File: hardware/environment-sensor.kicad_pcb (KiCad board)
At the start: 2 copper layers, 100 x 84 mm, 112 parts, among them J1 J1B1211CCD, P1 USB_OTG, P2 ICSP, P3 JTAG, P4 NSL-19M51, P5 PPD42, P6 POWER, SW1 Reset, U1 ATMEGA32U4-AU, U2 W5500, U3 Bosch_BME280, U4 LT1761-5, U5 LT1761-3.3, X1 16MHz, X2 25MHz

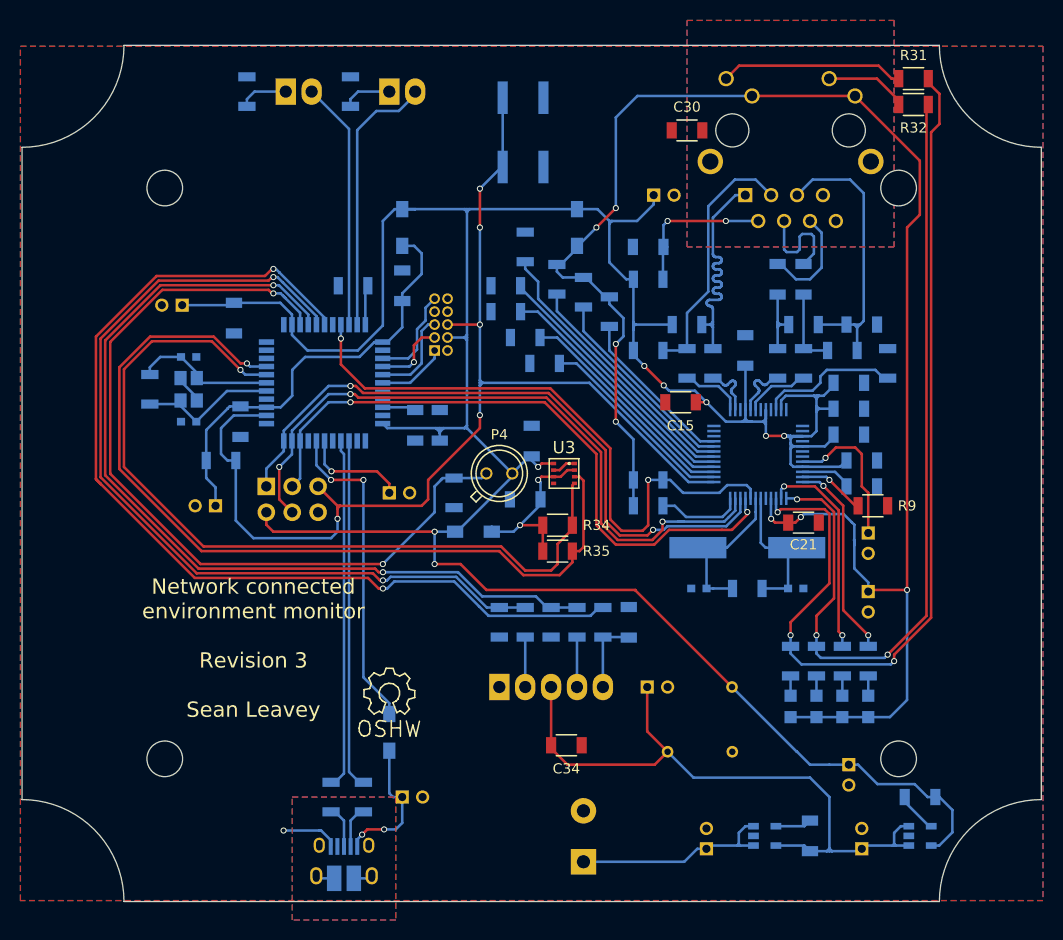
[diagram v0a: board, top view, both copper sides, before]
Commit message: New revision to board
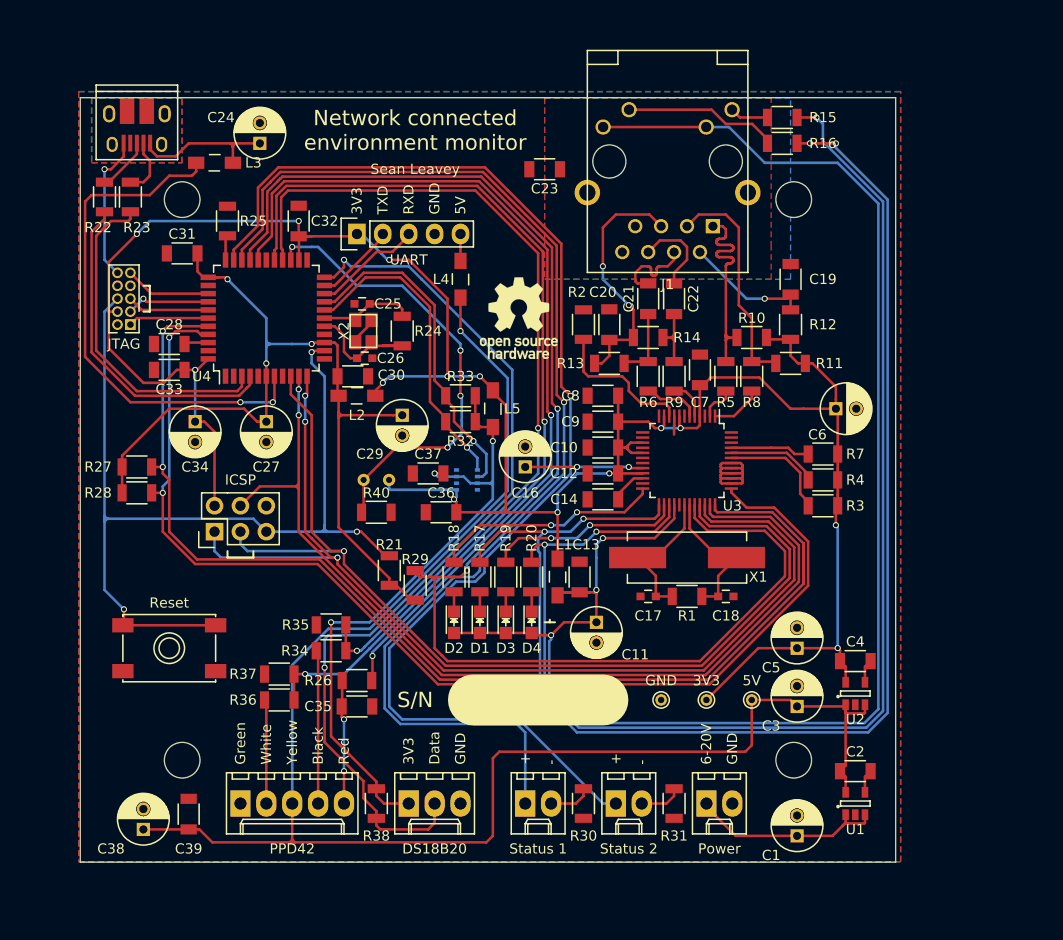
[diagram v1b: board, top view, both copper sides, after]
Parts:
- removed C15: 100n, Capacitors_SMD:C_1206
- removed D5: DUPLED, LEDs:LED_0805
- removed D6: ACTLED, LEDs:LED_0805
- removed R41, R42, R43: 330R, Resistors_SMD:R_1206
- removed REF**: Symbol_OSHW-Logo_SilkScreen, Symbols:Symbol_OSHW-Logo_SilkScreen
- removed the Ref** at (156.8, 101.0)
- added L5: Wurth WE-CBF, Choke_SMD:Choke_SMD_1206_Standard, F.Cu at (153.0, 94.6)
- added P7: JTAG, Pin_Headers:Pin_Header_Straight_2x05_Pitch1.27mm, F.Cu at (117.5, 86.4)
- added P8: DS18B20, Connectors_Molex:Molex_KK-6410-03_03x2.54mm_Straight, F.Cu at (144.8, 133.3)
- added P9: PPD42, Connectors_Molex:Molex_KK-6410-05_05x2.54mm_Straight, F.Cu at (128.3, 133.3)
- added REF***: OSHW-Logo_7.5x8mm_SilkScreen, Symbols:OSHW-Logo_7.5x8mm_SilkScreen, F.Cu at (155.6, 85.7)
- added Ref**: Val**, Board_Outlines:80mmx75mm_holes, F.Cu at (152.6, 101.6)
- C1, C10, C11, C12, C31, C32, C6, C7, C8, C9, L1, L2, L3, L4, R21, R36, R37, W1, W2, W3: moved to F.Cu
- C13, C33, C35, C37, C39: value 10u -> 100n; footprint Capacitors_ThroughHole:C_Radial_D5_L11_P2 -> Capacitors_SMD:C_1206; moved to F.Cu
- C14, C20: value 100n -> 10n; moved to F.Cu
- C16: value 100n -> 4u7; footprint Capacitors_SMD:C_1206 -> Capacitors_ThroughHole:C_Radial_D5_L11_P2; moved to F.Cu
- C17: value 100n -> 32p; footprint Capacitors_SMD:C_1206 -> Capacitors_SMD:C_0603; moved to F.Cu
- C18: value 10u -> 32p; footprint Capacitors_ThroughHole:C_Radial_D5_L11_P2 -> Capacitors_SMD:C_0603; moved to F.Cu
- C19: value 100n -> 22n; moved to F.Cu
- C2: value 12p -> 10n; footprint Capacitors_SMD:C_0603 -> Capacitors_SMD:C_1206; moved to F.Cu
- C21: value 100n -> 6.8n
- C22: value 10n -> 6.8n; moved to F.Cu
- C23: value 4u7 -> 1n/2kV; footprint Capacitors_ThroughHole:C_Radial_D5_L11_P2 -> Capacitors_SMD:C_1206; moved to F.Cu
- C24: value 32p -> 10u; footprint Capacitors_SMD:C_0603 -> Capacitors_ThroughHole:C_Radial_D5_L11_P2; moved to F.Cu
- C25: value 32p -> 12p; moved to F.Cu
- C26: value 22n -> 12p; footprint Capacitors_SMD:C_1206 -> Capacitors_SMD:C_0603; moved to F.Cu
- C27: value 10n -> 1u; footprint Capacitors_SMD:C_1206 -> Capacitors_ThroughHole:C_Radial_D5_L11_P2; moved to F.Cu
- C28: value 6.8n -> 100n; moved to F.Cu
- C29: value 6.8n -> 10u; footprint Capacitors_SMD:C_1206 -> Capacitors_ThroughHole:C_Radial_D5_L11_P2; moved to F.Cu
- C3: value 12p -> 10u; footprint Capacitors_SMD:C_0603 -> Capacitors_ThroughHole:C_Radial_D5_L11_P2; moved to F.Cu
- C30: value 1n/2kV -> 100n
- C34: value 100n -> 10u; footprint Capacitors_SMD:C_1206 -> Capacitors_ThroughHole:C_Radial_D5_L11_P2
- C36: value 10n -> 100n; moved to F.Cu
- C38: value 10n -> 10u; footprint Capacitors_SMD:C_1206 -> Capacitors_ThroughHole:C_Radial_D5_L11_P2; moved to F.Cu
- C4: value 1u -> 10n; footprint Capacitors_ThroughHole:C_Radial_D5_L11_P2 -> Capacitors_SMD:C_1206; moved to F.Cu
- C5: value 100n -> 10u; footprint Capacitors_SMD:C_1206 -> Capacitors_ThroughHole:C_Radial_D5_L11_P2; moved to F.Cu
- D1: value Status 1 -> LINKLED; footprint Connectors_Molex:Molex_KK-6410-02_02x2.54mm_Straight -> LEDs:LED_0805; moved to F.Cu
- D2: value Status 2 -> SPDLED; footprint Connectors_Molex:Molex_KK-6410-02_02x2.54mm_Straight -> LEDs:LED_0805; moved to F.Cu
- D3: value LINKLED -> DUPLED; moved to F.Cu
- D4: value SPDLED -> ACTLED; moved to F.Cu
- J1: footprint Cetus_RJ45:Cetus_J1B1211CCD -> Sockets_RJ45:Cetus_J1B1211CCD; moved to F.Cu
- P1: value USB_OTG -> POWER; footprint Connect:USB_Micro-B_10103594-0001LF -> Connectors_Molex:Molex_KK-6410-02_02x2.54mm_Straight; moved to F.Cu
- P2: value ICSP -> USB_OTG; footprint Pin_Headers:Pin_Header_Straight_2x03 -> Connect:USB_Micro-B_10103594-0001LF; moved to F.Cu
- P3: value JTAG -> ICSP; footprint Pin_Headers:Pin_Header_Straight_2x05_Pitch1.27mm -> Pin_Headers:Pin_Header_Straight_2x03; moved to F.Cu
- P4: value NSL-19M51 -> STATUS 1; footprint TO_SOT_Packages_THT:TO-18_2Pin -> Connectors_Molex:Molex_KK-6410-02_02x2.54mm_Straight
- P5: value PPD42 -> STATUS 2; footprint Connectors_Molex:Molex_KK-6410-05_05x2.54mm_Straight -> Connectors_Molex:Molex_KK-6410-02_02x2.54mm_Straight; moved to F.Cu
- P6: value POWER -> UART; footprint Terminal_Blocks:TerminalBlock_Pheonix_MKDS1.5-2pol -> Pin_Headers:Pin_Header_Straight_1x05; moved to F.Cu
- R1: value 10k -> 1M; moved to F.Cu
- R10, R11, R14: value 10k -> 49R9; moved to F.Cu
- R12: value 1M -> 10R; moved to F.Cu
- R13: value 12k4/1% -> 49R9; moved to F.Cu
- R15, R18, R19, R20: value 10k -> 330R; moved to F.Cu
- R16, R17: value 0R -> 330R; moved to F.Cu
- R2: value 22R -> 12k4/1%; moved to F.Cu
- R22, R23: value 10k -> 22R; moved to F.Cu
- R24: value 0R -> 1M; moved to F.Cu
- R25: value 0R -> 10k; moved to F.Cu
- R26, R27, R29: value 49R9/1% -> 10k; moved to F.Cu
- R28: value 10R/1% -> 10k; moved to F.Cu
- R3: value 22R -> 10k; moved to F.Cu
- R30: value 49R9/1% -> 180R; moved to F.Cu
- R31: value 330R -> 180R
- R32: value 330R -> 4k7
- R33, R38: value 10k -> 4k7; moved to F.Cu
- R34, R35: value 4k7 -> 10k
- R39: value 10k -> NSL-19M51; footprint Resistors_SMD:R_1206 -> LDRs_NSL:NSL_19M51
- R4: value 1M -> 10k; moved to F.Cu
- R40: value 330R -> 10k; moved to F.Cu
- R5, R8: value 10k -> 0R; moved to F.Cu
- R6: value 180R -> 0R; moved to F.Cu
- R7: value 180R -> 10k; moved to F.Cu
- R9: value 10k -> 0R
- SW1: value Reset -> RESET; footprint Buttons_Switches_SMD:SW_SPST_EVQP0 -> Buttons_Switches_SMD_FSM_JSM:SW_SPST_FSM_JSM; moved to F.Cu
- U1: value ATMEGA32U4-AU -> LT1761-5; footprint Housings_QFP:TQFP-44_10x10mm_Pitch0.8mm -> TO_SOT_Packages_SMD:SOT-23-5; moved to F.Cu
- U2: value W5500 -> LT1761-3.3; footprint Housings_QFP:LQFP-48_7x7mm_Pitch0.5mm -> TO_SOT_Packages_SMD:SOT-23-5; moved to F.Cu
- U3: value Bosch_BME280 -> W5500; footprint Bosch_Environment_Sensor:Bosch_BME280_LGA-8 -> Housings_QFP:LQFP-48_7x7mm_Pitch0.5mm
- U4: value LT1761-5 -> ATMEGA32U4-AU; footprint TO_SOT_Packages_SMD:SOT-23-5 -> Housings_QFP:TQFP-44_10x10mm_Pitch0.8mm; moved to F.Cu
- U5: value LT1761-3.3 -> Bosch_BME280; footprint TO_SOT_Packages_SMD:SOT-23-5 -> Sensors_LGA:Bosch_BME280_LGA-8
- X1: value 16MHz -> 25MHz; footprint Crystals:crystal_FA238-TSX3225 -> Crystals:Crystal_HC49-SD_SMD; moved to F.Cu
- X2: value 25MHz -> 16MHz; footprint Crystals:Crystal_HC49-SD_SMD -> Crystals:crystal_FA238-TSX3225; moved to F.Cu
- moved C2 77.0 mm to (188.6, 130.2), turned to 180 degrees
- moved C38 76.3 mm to (118.7, 135.9), turned to 90 degrees
- moved R31 74.9 mm to (170.8, 133.3), turned to 90 degrees
- moved U4 70.5 mm to (130.8, 85.7), turned to 90 degrees
- moved C24 68.3 mm to (130.2, 68.6), turned to 90 degrees
- moved R4 66.6 mm to (185.4, 101.6), turned to 180 degrees
- moved U1 66.4 mm to (188.6, 133.3)
- moved C3 65.9 mm to (182.9, 123.8), turned to 90 degrees
- moved P6 65.5 mm to (139.7, 77.5)
- moved C39 65.0 mm to (123.2, 134.4)
- moved C28 62.6 mm to (121.3, 88.3), turned to 180 degrees
- moved C6 61.6 mm to (186.7, 94.6), turned to 0 degrees
- moved SW1 61.4 mm to (121.3, 118.1), turned to 0 degrees
- moved C27 59.2 mm to (130.8, 95.9), turned to 270 degrees
- moved R7 58.4 mm to (185.4, 99.1), turned to 180 degrees
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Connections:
- C1 pad 1: Net-(C1-Pad1) -> /Power Supply/+6V
- C10 pad 1: GND -> /Microcontroller/3V3A
- C10 pad 2: /Microcontroller/3V3A -> GND
- C11 pad 1: /Microcontroller/3V3A -> /Network I/O/3V3D
- C12 pad 1: /Microcontroller/P_THRESH -> /Microcontroller/3V3A
- C13 pad 1: /Microcontroller/3V3A -> /Network I/O/3V3D
- C14 pad 1: /Microcontroller/3V3A -> GND
- C14 pad 2: GND -> Net-(C14-Pad2)
- C16 pad 1: /Microcontroller/3V3A -> Net-(C16-Pad1)
- C17 pad 1: /Microcontroller/3V3A -> GND
- C17 pad 2: GND -> Net-(C17-Pad2)
- C18 pad 1: /Network I/O/3V3D -> GND
- C18 pad 2: GND -> Net-(C18-Pad2)
- C19 pad 1: /Microcontroller/3V3A -> Net-(C19-Pad1)
- C2 pad 2: GND -> /Microcontroller/5VA
- C20 pad 1: /Microcontroller/3V3A -> Net-(C20-Pad1)
- C21 pad 1: /Network I/O/3V3D -> /Network I/O/RX2+
- C21 pad 2: GND -> /Network I/O/RX1+
- C22 pad 1: GND -> /Network I/O/RX2-
- C22 pad 2: Net-(C22-Pad2) -> /Network I/O/RX1-
- C23 pad 1: Net-(C23-Pad1) -> GND
- C23 pad 2: GND -> /Network I/O/CHGND
- C24 pad 1: GND -> Net-(C24-Pad1)
- C24 pad 2: Net-(C24-Pad2) -> GND
- C25 pad 1: GND -> Net-(C25-Pad1)
- C25 pad 2: Net-(C25-Pad2) -> GND
- C27 pad 1: Net-(C27-Pad1) -> /Microcontroller/3V3D
- C28 pad 1: /Network I/O/RX2+ -> Net-(C28-Pad1)
- C28 pad 2: /Network I/O/RX1+ -> GND
- C29 pad 1: /Network I/O/RX2- -> /Microcontroller/3V3D
- C29 pad 2: /Network I/O/RX1- -> GND
- C3 pad 1: Net-(C3-Pad1) -> /Microcontroller/5VA
- C30 pad 2: /Network I/O/CHGND -> /Microcontroller/3V3D
- C31 pad 1: /Microcontroller/3V3A -> GND
- C31 pad 2: GND -> /Microcontroller/3V3D
- C32 pad 1: /Sensors/3V3D -> GND
- C32 pad 2: GND -> /Microcontroller/3V3A
- C33 pad 1: /Power Supply/5VA -> GND
- C33 pad 2: GND -> /Microcontroller/3V3A
- C34 pad 1: GND -> /Microcontroller/3V3A
- C34 pad 2: /Power Supply/5VA -> GND
- C35 pad 1: /Power Supply/+6V -> /Microcontroller/DUST_2_THRESH
- C36 pad 1: Net-(C36-Pad1) -> /Microcontroller/3V3A
- C36 pad 2: /Power Supply/5VA -> GND
- C37 pad 1: /Power Supply/5VA -> /Sensors/3V3D
- C38 pad 1: Net-(C38-Pad1) -> /Microcontroller/5VA
- C38 pad 2: /Microcontroller/3V3A -> GND
- C39 pad 1: /Microcontroller/3V3A -> GND
- C39 pad 2: GND -> /Microcontroller/5VA
- C4 pad 2: GND -> /Microcontroller/3V3A
- C5 pad 1: Net-(C5-Pad1) -> /Microcontroller/3V3A
- C6 pad 1: /Microcontroller/3V3D -> /Microcontroller/3V3A
- C7 pad 1: GND -> /Microcontroller/3V3A
- C7 pad 2: /Microcontroller/3V3D -> GND
- C8 pad 1: GND -> /Microcontroller/3V3A
- C8 pad 2: /Microcontroller/3V3D -> GND
- C9 pad 1: GND -> /Microcontroller/3V3A
- C9 pad 2: /Microcontroller/3V3A -> GND
- D1 pad 2: Net-(D1-Pad2) -> /Network I/O/3V3D
- D2 pad 2: Net-(D2-Pad2) -> /Network I/O/3V3D
- J1 pad 2: Net-(C26-Pad1) -> Net-(C19-Pad1)
- J1 pad 5: Net-(C27-Pad1) -> Net-(C20-Pad1)
- L1 pad 1: /Microcontroller/3V3A -> /Network I/O/3V3D
- L1 pad 2: /Microcontroller/3V3D -> /Microcontroller/3V3A
- L2 pad 1: Net-(C1-Pad1) -> /Microcontroller/3V3A
- L2 pad 2: Net-(L2-Pad2) -> /Microcontroller/3V3D
- L3 pad 1: /Microcontroller/3V3A -> Net-(C24-Pad1)
- L3 pad 2: /Network I/O/3V3D -> Net-(L3-Pad2)
- L4 pad 1: /Microcontroller/3V3A -> Net-(L4-Pad1)
- L4 pad 2: /Sensors/3V3D -> /Microcontroller/5VA
- P1 pad 1: Net-(C1-Pad1) -> /Power Supply/+6V
- P1 pad 2: /Microcontroller/USBD- -> GND
- P2 pad 1: /Microcontroller/SPI_MISO -> Net-(C24-Pad1)
- P2 pad 2: /Microcontroller/3V3A -> /Microcontroller/USBD-
- P2 pad 3: /Microcontroller/SPI_SCLK -> /Microcontroller/USBD+
- P2 pad 4: /Microcontroller/SPI_MOSI -> (no net)
- P2 pad 5: /Microcontroller/~RESET -> GND
- P2 pad 6: GND -> Net-(P2-Pad6)
- P3 pad 1: Net-(P3-Pad1) -> /Microcontroller/SPI_MISO
- P3 pad 2: GND -> /Microcontroller/3V3A
- P3 pad 3: Net-(P3-Pad3) -> /Microcontroller/SPI_SCLK
- P3 pad 4: /Microcontroller/3V3A -> /Microcontroller/SPI_MOSI
- P3 pad 5: Net-(P3-Pad5) -> /Microcontroller/~RESET
- P3 pad 6: /Microcontroller/~RESET -> GND
- P4 pad 1: /Microcontroller/3V3A -> /Microcontroller/STATUS_1
- P4 pad 2: /Microcontroller/LDR_OUT -> Net-(P4-Pad2)
- P5 pad 1: GND -> /Microcontroller/STATUS_2
- P6 pad 1: /Power Supply/+6V -> /Microcontroller/3V3A
- P6 pad 2: GND -> Net-(P6-Pad2)
- R1 pad 1: /Microcontroller/3V3D -> Net-(C17-Pad2)
- R1 pad 2: /Microcontroller/~RESET -> Net-(C18-Pad2)
- R10 pad 1: /Network I/O/3V3D -> /Network I/O/TX1+
- R10 pad 2: /Microcontroller/SS_PHY -> /Microcontroller/3V3A
- R11 pad 1: /Network I/O/3V3D -> /Network I/O/TX1-
- R11 pad 2: Net-(R11-Pad2) -> /Microcontroller/3V3A
- R12 pad 1: Net-(C24-Pad2) -> Net-(C19-Pad1)
- R12 pad 2: Net-(C25-Pad2) -> /Microcontroller/3V3A
- R13 pad 1: GND -> Net-(C20-Pad1)
- R13 pad 2: Net-(R13-Pad2) -> /Network I/O/RX1+
- R14 pad 1: /Network I/O/3V3D -> Net-(C20-Pad1)
- R14 pad 2: Net-(R14-Pad2) -> /Network I/O/RX1-
- R15 pad 1: /Network I/O/3V3D -> Net-(J1-Pad9)
- R15 pad 2: Net-(R15-Pad2) -> /Network I/O/ACTLED
- R16 pad 1: /Network I/O/TX1+ -> Net-(J1-Pad11)
- R16 pad 2: /Network I/O/TX+ -> /Network I/O/LINKLED
- R17 pad 1: /Network I/O/RX1+ -> Net-(D1-Pad1)
- R17 pad 2: /Network I/O/RX+ -> /Network I/O/LINKLED
- R18 pad 1: GND -> Net-(D2-Pad1)
- R18 pad 2: Net-(R18-Pad2) -> /Network I/O/SPDLED
- R19 pad 1: GND -> Net-(D3-Pad1)
- R19 pad 2: Net-(R19-Pad2) -> /Network I/O/DUPLED
- R2 pad 1: /Microcontroller/USBD1+ -> GND
- R2 pad 2: /Microcontroller/USBD+ -> Net-(R2-Pad2)
- R20 pad 1: GND -> Net-(D4-Pad1)
- R20 pad 2: Net-(R20-Pad2) -> /Network I/O/ACTLED
- R21 pad 1: GND -> /Microcontroller/~RESET
- R21 pad 2: Net-(R21-Pad2) -> /Microcontroller/3V3D
- R22 pad 1: GND -> /Microcontroller/USBD+
- R22 pad 2: Net-(R22-Pad2) -> /Microcontroller/USBD1+
- R23 pad 1: /Network I/O/3V3D -> /Microcontroller/USBD-
- R23 pad 2: Net-(R23-Pad2) -> /Microcontroller/USBD1-
- R24 pad 1: /Network I/O/TX1- -> Net-(C26-Pad1)
- R24 pad 2: /Network I/O/TX- -> Net-(C25-Pad1)
- R25 pad 1: /Network I/O/RX1- -> Net-(R25-Pad1)
- R25 pad 2: /Network I/O/RX- -> GND
- R26 pad 1: /Network I/O/TX1+ -> /Microcontroller/DUST_2_THRESH
- R26 pad 2: /Microcontroller/3V3A -> Net-(R26-Pad2)
- R27 pad 1: /Network I/O/TX1- -> /Microcontroller/~PHY_INTERRUPT
- R27 pad 2: /Microcontroller/3V3A -> /Microcontroller/3V3D
- R28 pad 1: Net-(C26-Pad1) -> /Microcontroller/~PHY_RESET
- R28 pad 2: /Microcontroller/3V3A -> /Microcontroller/3V3D
- R29 pad 1: Net-(C27-Pad1) -> /Microcontroller/PHY_SS
- R29 pad 2: /Network I/O/RX1+ -> /Microcontroller/3V3D
- R3 pad 1: /Microcontroller/USBD1- -> /Microcontroller/3V3A
- R3 pad 2: /Microcontroller/USBD- -> Net-(R3-Pad2)
- R30 pad 1: Net-(C27-Pad1) -> GND
- R30 pad 2: /Network I/O/RX1- -> Net-(P4-Pad2)
- R31 pad 1: Net-(J1-Pad9) -> GND
- R31 pad 2: /Network I/O/ACTLED -> Net-(P5-Pad2)
- R32 pad 1: Net-(J1-Pad11) -> /Sensors/3V3D
- R32 pad 2: /Network I/O/LINKLED -> /Microcontroller/I2C_SCLK
- R33 pad 1: /Microcontroller/LDR_OUT -> /Sensors/3V3D
- R33 pad 2: GND -> /Microcontroller/I2C_SDA
- R34 pad 1: /Sensors/3V3D -> /Microcontroller/DUST_1
- R34 pad 2: /Microcontroller/I2C_SCLK -> Net-(P9-Pad4)
- R35 pad 1: /Sensors/3V3D -> GND
- R35 pad 2: /Microcontroller/I2C_SDA -> /Microcontroller/DUST_1
- R36 pad 1: /Microcontroller/P_OUT_1 -> /Microcontroller/DUST_2
- R36 pad 2: Net-(P5-Pad4) -> Net-(P9-Pad2)
- R37 pad 2: /Microcontroller/P_OUT_1 -> /Microcontroller/DUST_2
- R38 pad 1: /Microcontroller/P_OUT_2 -> /Microcontroller/DS18B20
- R38 pad 2: Net-(P5-Pad2) -> /Sensors/3V3D
- R39 pad 1: GND -> /Microcontroller/LDR
- R39 pad 2: /Microcontroller/P_OUT_2 -> /Microcontroller/3V3A
- R4 pad 1: Net-(C2-Pad1) -> /Microcontroller/3V3A
- R4 pad 2: Net-(C3-Pad1) -> Net-(R4-Pad2)
- R40 pad 1: Net-(D3-Pad1) -> /Microcontroller/LDR
- R40 pad 2: /Network I/O/LINKLED -> GND
- R5 pad 1: GND -> /Network I/O/TX1+
- R5 pad 2: Net-(R5-Pad2) -> /Network I/O/TX+
- R6 pad 1: GND -> /Network I/O/RX1+
- R6 pad 2: Net-(D1-Pad1) -> /Network I/O/RX+
- R7 pad 1: GND -> /Microcontroller/3V3A
- R7 pad 2: Net-(D2-Pad1) -> Net-(R7-Pad2)
- R8 pad 1: /Microcontroller/P_THRESH -> /Network I/O/TX1-
- R8 pad 2: Net-(R8-Pad2) -> /Network I/O/TX-
- R9 pad 1: Net-(R9-Pad1) -> /Network I/O/RX1-
- R9 pad 2: GND -> /Network I/O/RX-
- U1 pad 1: (no net) -> /Power Supply/+6V
- U1 pad 2: (no net) -> GND
- U1 pad 3: /Microcontroller/USBD1- -> /Power Supply/+6V
- U1 pad 4: /Microcontroller/USBD1+ -> Net-(C2-Pad1)
- U1 pad 5: GND -> /Microcontroller/5VA
- U2 pad 1: /Network I/O/TX- -> /Microcontroller/5VA
- U2 pad 2: /Network I/O/TX+ -> GND
- U2 pad 3: GND -> /Microcontroller/5VA
- U2 pad 4: /Microcontroller/3V3A -> Net-(C4-Pad1)
- U2 pad 5: /Network I/O/RX- -> /Microcontroller/3V3A
- U3 pad 1: GND -> /Network I/O/TX-
- U3 pad 2: /Sensors/3V3D -> /Network I/O/TX+
- U3 pad 3: /Microcontroller/I2C_SDA -> GND
- U3 pad 4: /Microcontroller/I2C_SCLK -> /Microcontroller/3V3A
- U3 pad 5: GND -> /Network I/O/RX-
- U3 pad 6: /Sensors/3V3D -> /Network I/O/RX+
- U3 pad 7: GND -> (no net)
- U4 pad 1: /Power Supply/+6V -> (no net)
- U4 pad 2: GND -> (no net)
- U4 pad 3: /Power Supply/+6V -> /Microcontroller/USBD1-
- U4 pad 4: Net-(C36-Pad1) -> /Microcontroller/USBD1+
- U4 pad 5: /Power Supply/5VA -> GND
- U5 pad 1: /Power Supply/5VA -> GND
- U5 pad 2: GND -> /Sensors/3V3D
- U5 pad 3: /Power Supply/5VA -> /Microcontroller/I2C_SDA
- U5 pad 4: Net-(C38-Pad1) -> /Microcontroller/I2C_SCLK
- U5 pad 5: /Microcontroller/3V3A -> GND
- W1 pad 1: /Power Supply/5VA -> /Microcontroller/5VA
- X1 pad 1: Net-(C2-Pad1) -> Net-(C18-Pad2)
- X1 pad 2: Net-(C3-Pad1) -> Net-(C17-Pad2)
- X2 pad 1: Net-(C25-Pad2) -> Net-(C25-Pad1)
- X2 pad 2: Net-(C24-Pad2) -> Net-(C26-Pad1)
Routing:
- net /Microcontroller/5VA: track 0.00 -> 162.5 mm, vias 0 -> 1
- net /Microcontroller/PHY_SS: track 0.00 -> 141.4 mm, vias 0 -> 2
- net /Microcontroller/STATUS_2: track 0.00 -> 122.2 mm, vias 0 -> 1
- net /Microcontroller/~PHY_INTERRUPT: track 0.00 -> 118.2 mm, vias 0 -> 2
- net /Microcontroller/STATUS_1: track 0.00 -> 116.1 mm, vias 0 -> 1
- net /Microcontroller/~PHY_RESET: track 0.00 -> 112.4 mm, vias 0 -> 2
- net Net-(R8-Pad2): track 98.7 -> 0.00 mm, vias 2 -> 0
- net /Microcontroller/DUST_2: track 0.00 -> 92.7 mm, vias 0 -> 2
- net /Microcontroller/P_OUT_1: track 89.2 -> 0.00 mm, vias 2 -> 0
- net /Microcontroller/DS18B20: track 0.00 -> 88.9 mm, vias 0 -> 2
- net Net-(R26-Pad2): track 0.00 -> 87.1 mm, vias 0 -> 2
- net /Microcontroller/P_OUT_2: track 87.0 -> 0.00 mm, vias 2 -> 0
- net /Microcontroller/DUST_1: track 0.00 -> 84.5 mm, vias 0 -> 2
- net /Microcontroller/LDR_OUT: track 82.1 -> 0.00 mm, vias 2 -> 0
- net /Power Supply/5VA: track 66.5 -> 0.00 mm
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- added copper zone on B.Cu, net Net-(P2-Pad6)
- added copper zone on F.Cu, net Net-(P2-Pad6)
- removed copper zone on B.Cu, net Net-(P1-Pad6)
- removed copper zone on F.Cu, net Net-(P1-Pad6)
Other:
- board size 100 x 84 mm -> 80 x 75 mm
- board text added: "+"
- board text added: "-"
- board text added: "3V3"
- board text added: "6-20V"
- board text added: "DS18B20"
- board text added: "Data"
- board text added: "Network connected environment monitor"
- board text added: "Power"
- board text added: "RXD"
- board text added: "S/N"
- board text added: "Sean Leavey"
- board text added: "TXD"
- board text added: "UART"
- board text removed: "3.3V"
- board text removed: "6V"
- board text removed: "Network connected environment monitor Revision 3 Sean Leavey"
- board text removed: "S/N:"
